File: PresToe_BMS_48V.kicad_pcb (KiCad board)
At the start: 2 copper layers, 45 parts, among them J1 XT90PB-F, J2 XT90PB-F, J3 XT30PW-M, J4 S3B-XH-A, J5 Conn_01x06_Pin, P1 T93YA203JT20, Q1 IAUS200N08S5N023ATMA1, Q2 IAUS200N08S5N023ATMA1, Q3 IAUS200N08S5N023ATMA1, SW1 DS04-254-1-01BK-SMT, U1 PTPS48000QDGXRQ1, U2 TPSM265R1SILR, U3 INA241A2QDGKRQ1, U4 TLV9051IDBVR, U5 MCP3202T-CI/MS, U6 ISO6741DWR

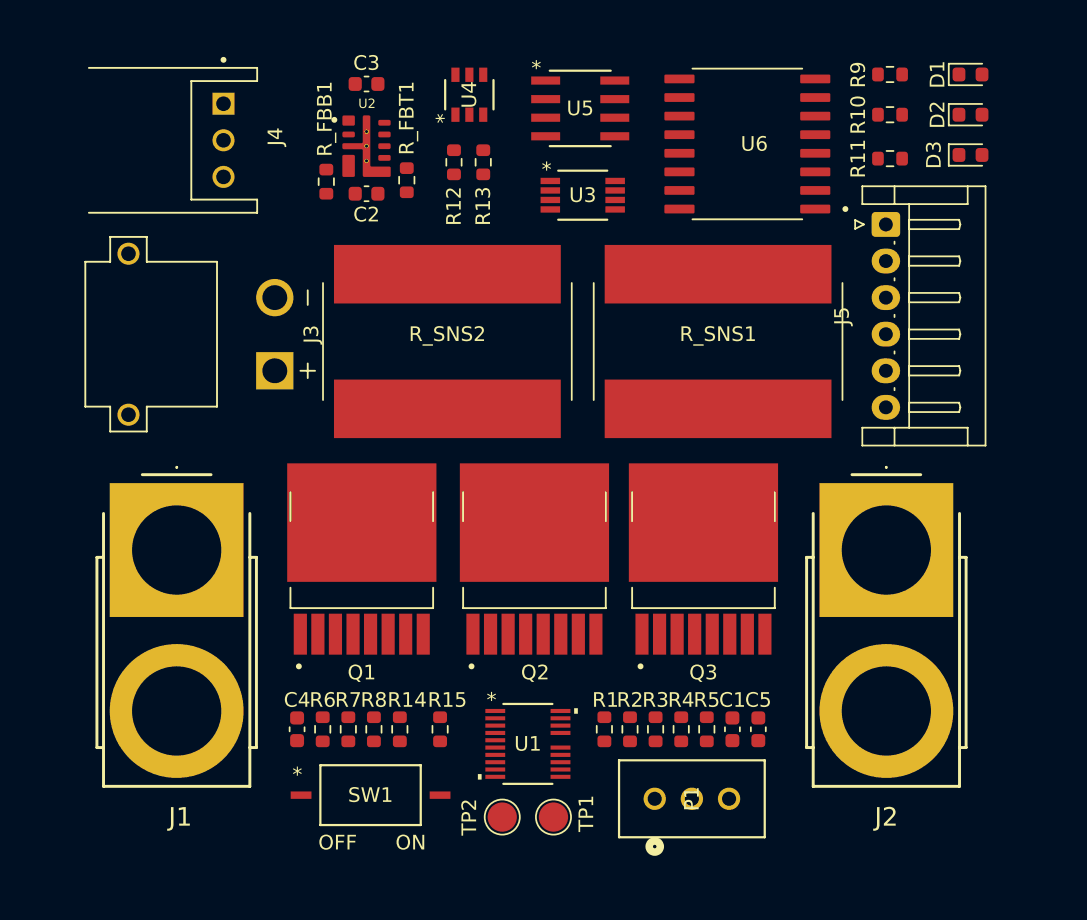
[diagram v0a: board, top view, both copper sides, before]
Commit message: finalized, remaining final checks
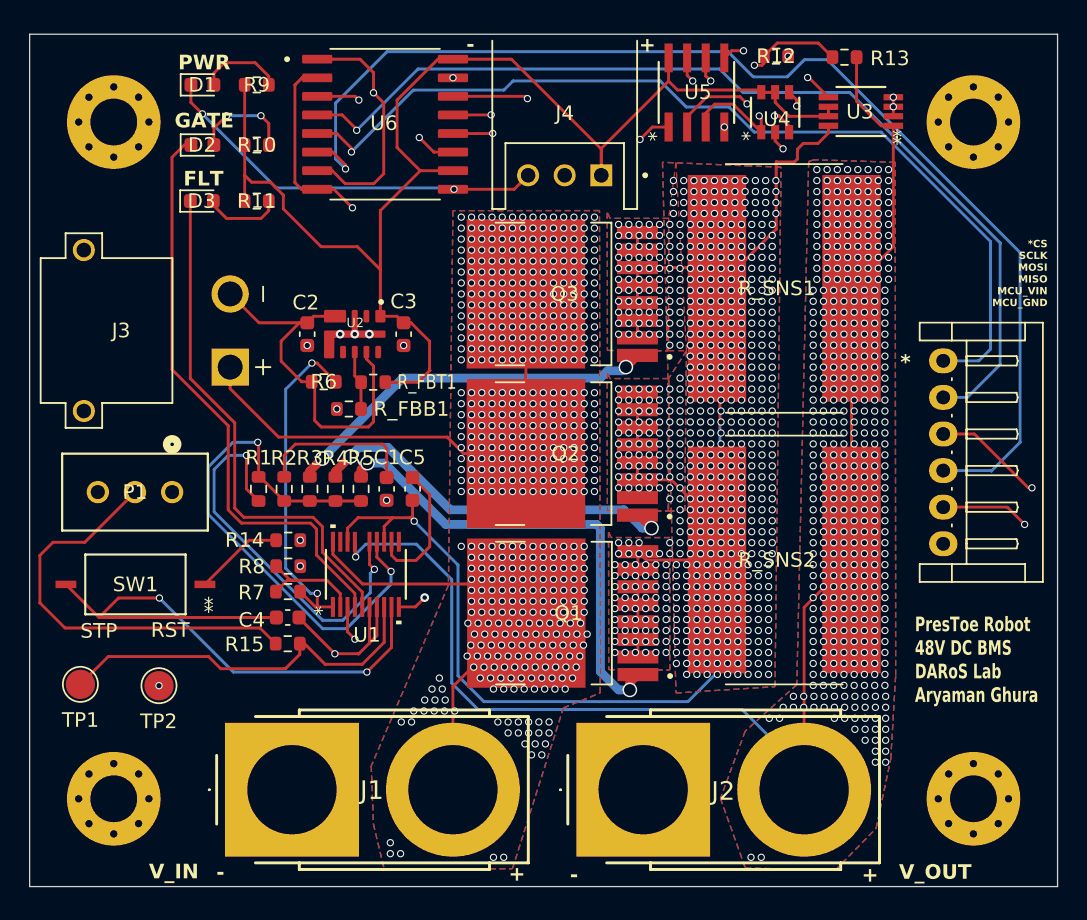
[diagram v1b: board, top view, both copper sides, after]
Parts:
- added H1: MountingHole, MountingHole:MountingHole_3.2mm_M3_Pad_Via, F.Cu at (34.2, 32.0)
- added H2: MountingHole, MountingHole:MountingHole_3.2mm_M3_Pad_Via, F.Cu at (93.0, 32.0)
- added H3: MountingHole, MountingHole:MountingHole_3.2mm_M3_Pad_Via, F.Cu at (34.2, 78.2)
- added H4: MountingHole, MountingHole:MountingHole_3.2mm_M3_Pad_Via, F.Cu at (93.0, 78.2)
- moved D3 52.6 mm to (40.3, 37.4)
- moved D2 52.5 mm to (40.3, 33.6)
- moved D1 52.5 mm to (40.3, 29.5)
- moved R11 43.4 mm to (44.0, 37.4)
- moved R10 43.3 mm to (44.0, 33.6)
- moved R9 43.3 mm to (44.0, 29.5)
- moved P1 39.1 mm to (38.2, 57.3), turned to -90 degrees
- moved TP1 33.6 mm to (32.0, 70.4)
- moved J4 29.2 mm to (65.1, 29.9), turned to 180 degrees
- moved C1 28.8 mm to (52.9, 57.1)
- moved C5 28.8 mm to (54.7, 57.1), turned to 90 degrees
- moved R1 28.8 mm to (44.1, 57.1)
- moved R2 28.8 mm to (45.9, 57.1)
- moved R3 28.8 mm to (47.6, 57.1)
- moved R4 28.8 mm to (49.4, 57.1)
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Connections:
- U4 pad 1: Net-(U4-OUT) -> Net-(U4--IN)
- U4 pad 4: V_ADC -> Net-(U4--IN)
- U5 pad 3: Net-(U4-OUT) -> Net-(U4--IN)
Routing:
- net V_out: track 0.00 -> 120.1 mm, vias 0 -> 654
- net SPI_VIN: track 0.00 -> 102.8 mm, vias 0 -> 2
- net V_load: track 0.00 -> 96.9 mm, vias 0 -> 427
- net 5V: track 0.00 -> 90.8 mm
- net SPI_GND: track 0.00 -> 87.7 mm, vias 0 -> 1
- net SPI_MISO: track 0.00 -> 81.3 mm, vias 0 -> 1
- net INP: track 0.00 -> 80.0 mm, vias 0 -> 1
- net SPI_MOSI: track 0.00 -> 78.7 mm, vias 0 -> 2
- net SPI_SCLK: track 0.00 -> 66.9 mm, vias 0 -> 1
- net SPI_*CS: track 0.00 -> 64.3 mm, vias 0 -> 1
- net V_in: track 0.00 -> 61.5 mm, vias 0 -> 532
- net GND: track 0.00 -> 61.3 mm, vias 0 -> 20
- net Net-(U1-TMR): track 0.00 -> 41.4 mm, vias 0 -> 2
- net FLT_GD: track 0.00 -> 40.3 mm
- net Net-(U1-PD): track 0.00 -> 37.6 mm, vias 0 -> 2
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- added copper zone on In1.Cu, net GND
- added copper zone on B.Cu, net V_in
- added copper zone on F.Cu, net V_in
- added copper zone on In2.Cu, net V_in
- added copper zone on In3.Cu, net V_in
- added copper zone on In4.Cu, net V_in
- added copper zone on B.Cu, net V_load
- added copper zone on F.Cu, net V_load
- added copper zone on In2.Cu, net V_load
- added copper zone on In3.Cu, net V_load
- added copper zone on In4.Cu, net V_load
- added copper zone on B.Cu, net V_out
- added copper zone on F.Cu, net V_out
- added copper zone on In2.Cu, net V_out
- added copper zone on In3.Cu, net V_out
- added copper zone on In4.Cu, net V_out
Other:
- board outline added: 70.2 x 58.2 mm
- copper layers 2 -> 6
- board text added: "*"
- board text added: "*CS SCLK MOSI MISO MCU_VIN MCU_GND"
- board text added: "+"
- board text added: "-"
- board text added: "FLT"
- board text added: "GATE"
- board text added: "PWR"
- board text added: "PresToe Robot 48V DC BMS DARoS Lab Aryaman Ghura"
- board text added: "V_IN"
- board text added: "V_OUT"
